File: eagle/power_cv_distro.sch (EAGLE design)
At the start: 54 parts, among them U1 POWER, U10 TLV2372IP, U11 TLV2372IP, U12 TLV2372IP, U13 TLV2372IP, U2 POWER, U3 POWER, U4 POWER, U5 POWER, U6 POWER, U7 POWER, U8 POWER, U9 POWER

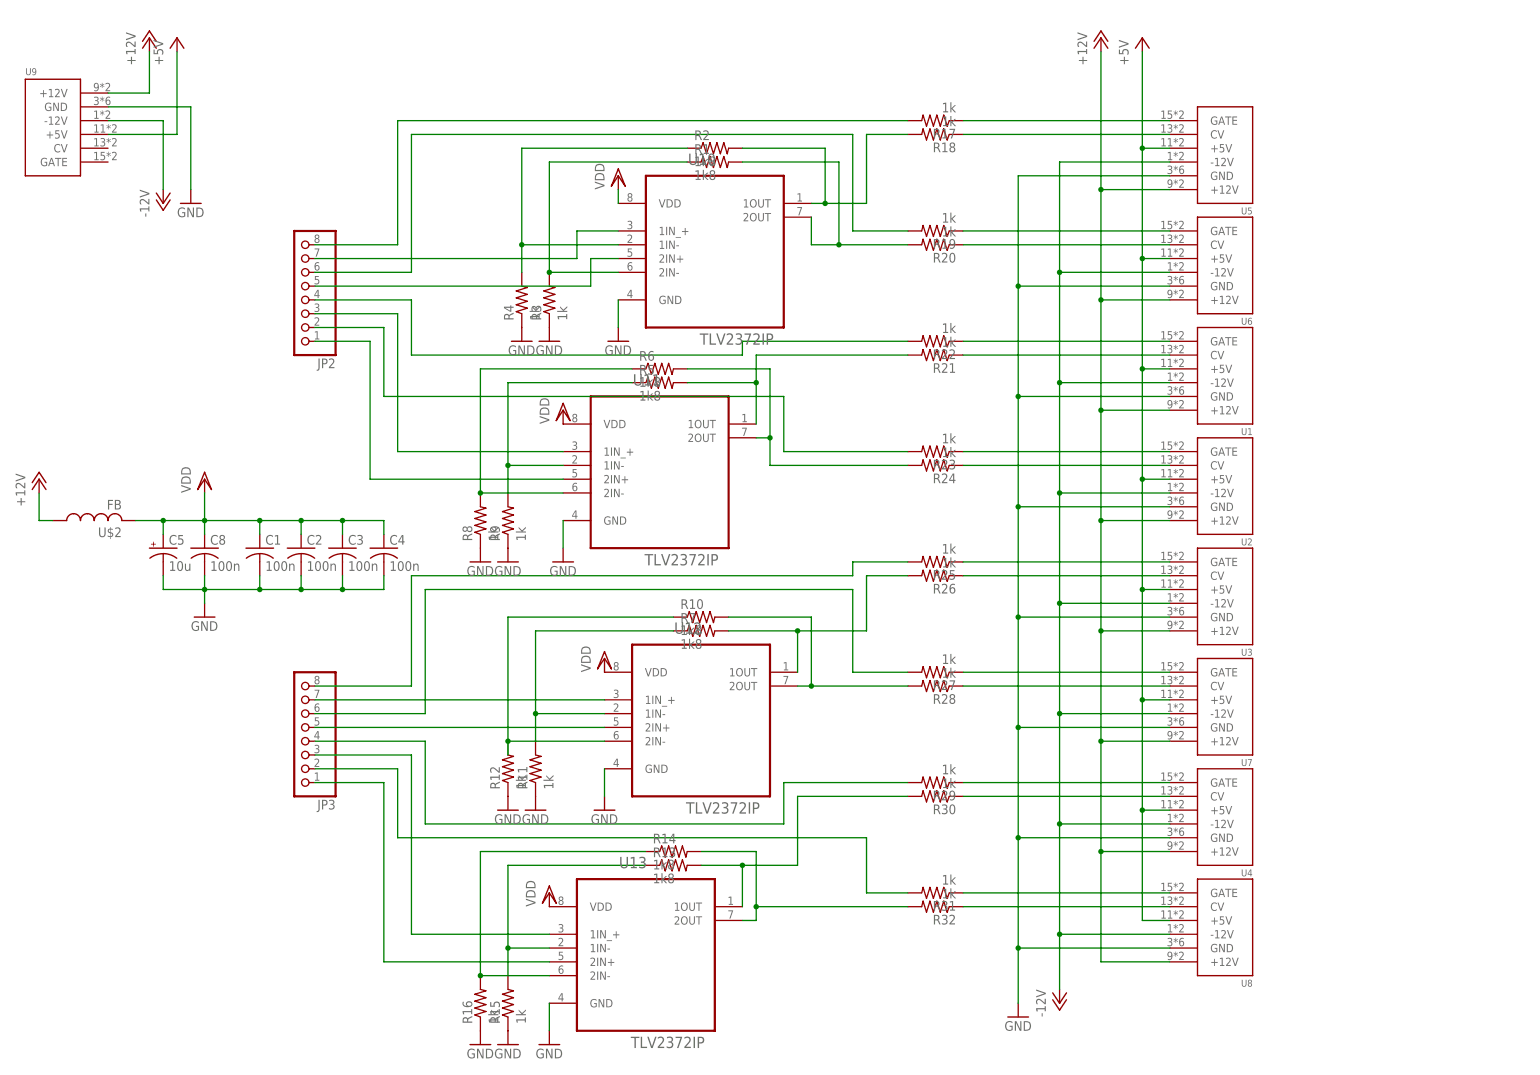
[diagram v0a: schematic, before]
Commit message: power dist do-over begins
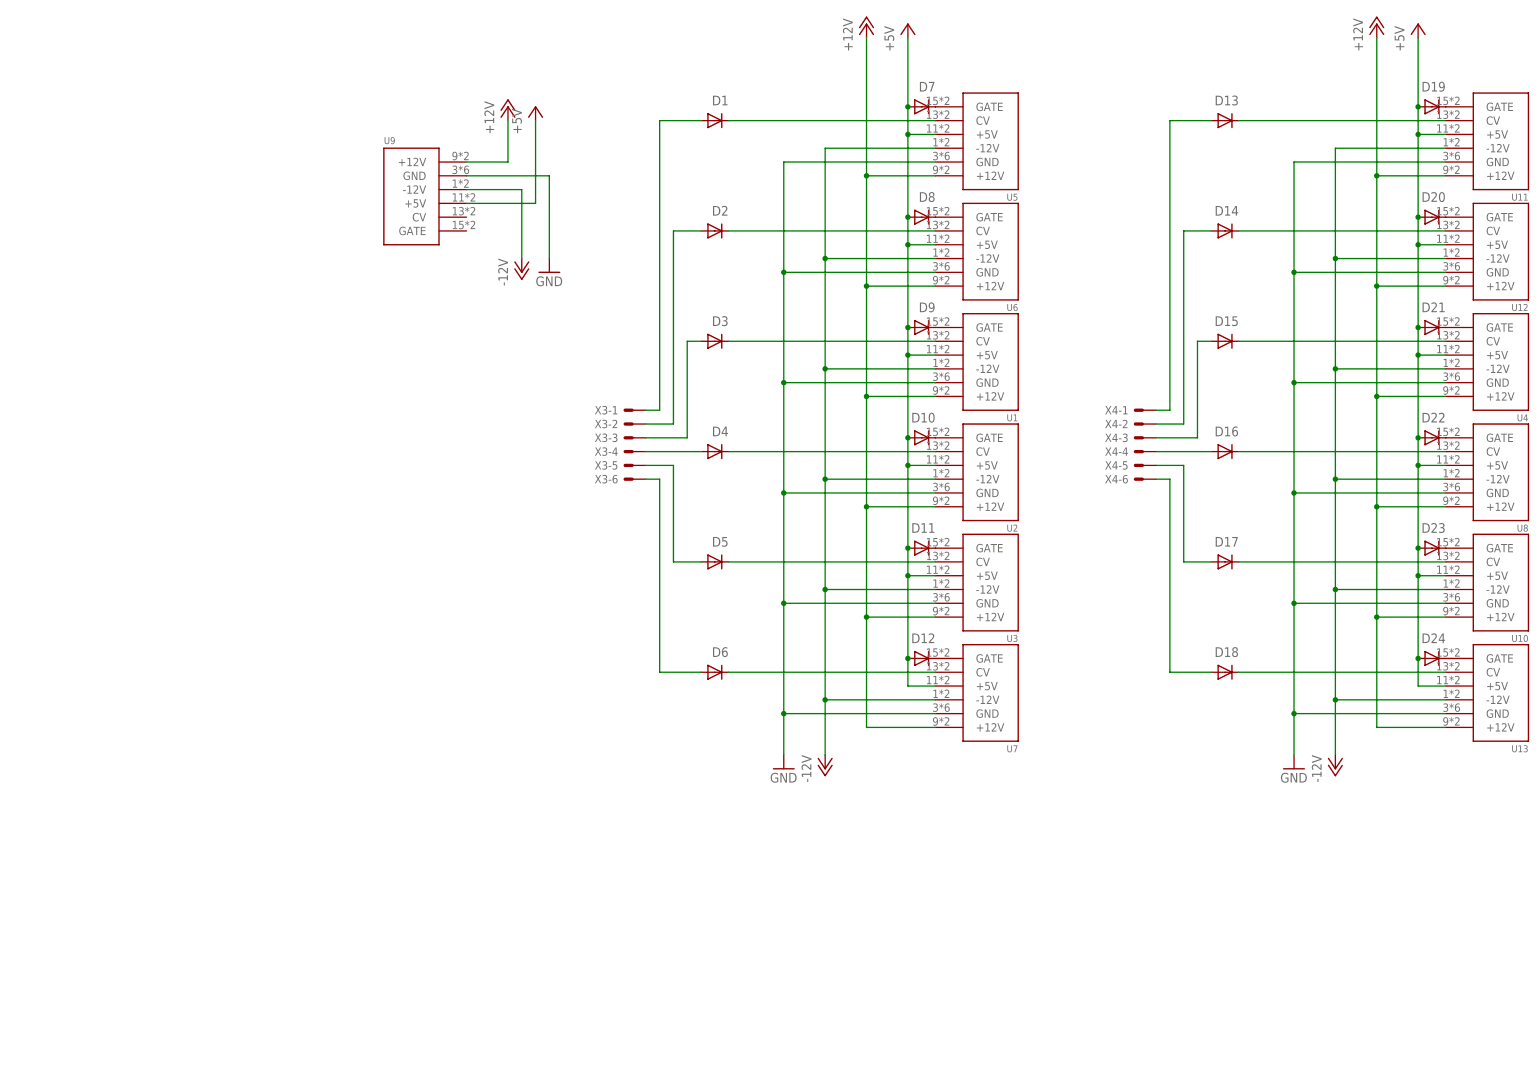
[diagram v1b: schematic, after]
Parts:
- removed C1, C2, C3, C4: 100n, rcl:C-US025-025X050
- removed C5: 10u, rcl:CPOL-USB45181A
- removed C8: 100n, rcl:C-US050-024X044
- removed JP2, JP3: (no value), pinhead:PINHD-1X8
- removed R1, R10, R13, R14, R2, R5, R6, R7: 1k8, rcl:R-US_0204/2V
- removed R11, R12, R15, R16, R17, R18, R19, R20, R21, R22, R23, R24, R25, R26, R27, R28, R29, R3, R30, R31, R32, R4, R8, R9: 1k, rcl:R-US_0207/7
- removed U$2: FB, adafruit:FB
- added D1, D10, D11, D12, D13, D14, D15, D16, D17, D18, D19, D2, D20, D21, D22, D23, D24, D3, D4, D5, D6, D7, D8, D9: 1N4148DO35-7, TR808clone:1N4148DO35-7
- added X3, X4: (no value), con-molex:22-23-2061
- U10, U11, U12, U13: value TLV2372IP -> POWER; device Texas Instruments_By_element14_Batch_1:TLV2372IP -> eurorack:POWER
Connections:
- removed net N$37: R22.1, U1.GATE
- removed net N$38: R21.1, U1.CV
- removed net N$39: R23.1, U2.GATE
- removed net N$40: R24.1, U2.CV
- removed net N$41: R25.1, U3.GATE
- removed net N$42: R26.1, U3.CV
- removed net N$43: R27.1, U7.GATE
- removed net N$44: R28.1, U7.CV
- removed net N$45: R29.1, U4.GATE
- removed net N$46: R30.1, U4.CV
- removed net N$47: R31.1, U8.GATE
- removed net N$48: R32.1, U8.CV
- removed net VDD: C1.1, C2.1, C3.1, C4.1, C5.+, C8.1, U$2.2, U10.VDD, U11.VDD, U12.VDD, U13.VDD
- net +12V: no longer U$2.1
- net +5V: now also D10.A, D11.A, D12.A, D19.A, D20.A, D21.A, D22.A, D23.A, D24.A, D7.A, D8.A, D9.A, U10.+5V, U11.+5V, U12.+5V, U13.+5V
- net -12V: now also U10.-12V, U11.-12V, U12.-12V, U13.-12V
- net GND: no longer C1.2, C2.2, C3.2, C4.2, C5.-, C8.2, R11.1, R12.1, R15.1, R16.1, R3.1, R4.1, R8.1, R9.1
- net N$1: now also D1.A, X3-1.S; no longer JP2.8, R17.2
- net N$10: now also D4.C, U2.CV; no longer JP3.7, U12.1IN_+
- net N$11: now also D5.C, U3.CV; no longer JP3.6, R27.2
- net N$12: now also D6.C, U7.CV; no longer JP3.5, U12.2IN+
- net N$13: now also D7.C, U5.GATE; no longer JP3.4, R29.2
- net N$14: now also D8.C, U6.GATE; no longer R10.2, R28.2, U12.2OUT
- net N$15: now also D9.C, U1.GATE; no longer JP3.2, R31.2
- net N$16: now also D10.C, U2.GATE; no longer JP3.1, U13.2IN+
- net N$17: now also D11.C, U3.GATE; no longer R1.2, R20.2, U10.2OUT
- net N$18: now also D12.C, U7.GATE; no longer R18.2, R2.2, U10.1OUT
- net N$19: now also D13.A, X4-1.S; no longer R1.1, R3.2, U10.2IN-
- net N$2: now also D2.A, X3-2.S; no longer JP2.7, U10.1IN_+
- net N$20: now also D14.A, X4-2.S; no longer R2.1, R4.2, U10.1IN-
- net N$21: now also D15.A, X4-3.S; no longer R11.2, R7.1, U12.1IN-
- net N$22: now also D17.A, X4-5.S; no longer R24.2, R6.2, U11.2OUT
- net N$23: now also D18.A, X4-6.S; no longer R5.1, R9.2, U11.1IN-
- net N$24: now also D16.A, X4-4.S; no longer R6.1, R8.2, U11.2IN-
- net N$25: now also D13.C, U11.CV; no longer R10.1, R12.2, U12.2IN-
- net N$26: now also D14.C, U12.CV; no longer R21.2, R5.2, U11.1OUT
- net N$27: now also D15.C, U4.CV; no longer R26.2, R7.2, U12.1OUT
- net N$28: now also D16.C, U8.CV; no longer R13.2, R30.2, U13.1OUT
- net N$29: now also D17.C, U10.CV; no longer R14.2, R32.2, U13.2OUT
- net N$3: now also D3.A, X3-3.S; no longer JP2.6, R19.2
- net N$30: now also D18.C, U13.CV; no longer JP3.3, U13.1IN_+
- net N$31: now also D19.C, U11.GATE; no longer R13.1, R15.2, U13.1IN-
- net N$32: now also D20.C, U12.GATE; no longer R14.1, R16.2, U13.2IN-
- net N$33: now also D21.C, U4.GATE; no longer R17.1, U5.GATE
- net N$34: now also D22.C, U8.GATE; no longer R18.1, U5.CV
- net N$35: now also D23.C, U10.GATE; no longer R20.1, U6.CV
- net N$36: now also D24.C, U13.GATE; no longer R19.1, U6.GATE
- net N$4: now also D4.A, X3-4.S; no longer JP2.5, U10.2IN+
- net N$49: now also U10.+12V, U11.+12V, U12.+12V, U13.+12V
- net N$5: now also D5.A, X3-5.S; no longer JP2.4, R22.2
- net N$6: now also D6.A, X3-6.S; no longer JP2.3, U11.1IN_+
- net N$7: now also D1.C, U5.CV; no longer JP2.2, R23.2
- net N$8: now also D2.C, U6.CV; no longer JP2.1, U11.2IN+
- net N$9: now also D3.C, U1.CV; no longer JP3.8, R25.2
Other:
- moved on the sheet: U1, U2, U3, U4, U5, U6, U7, U8, U9
